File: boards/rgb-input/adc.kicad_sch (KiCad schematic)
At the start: 1 part, among them U2 MCP3208

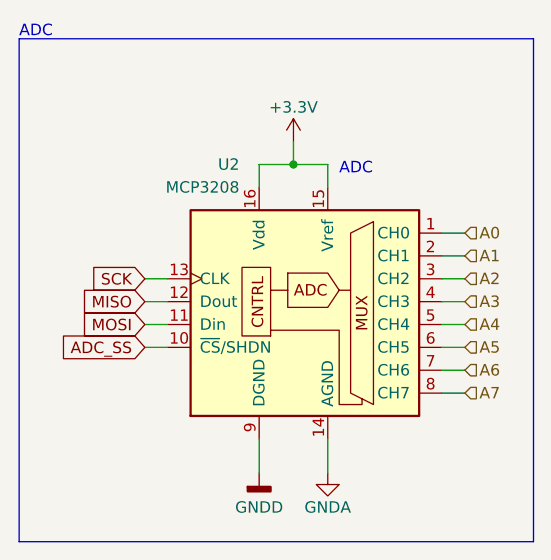
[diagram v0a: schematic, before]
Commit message: new rgb input board is starting to look very nice.
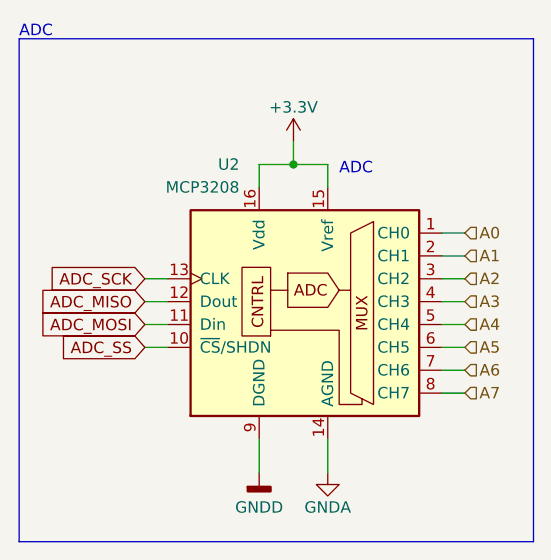
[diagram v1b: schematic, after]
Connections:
- net MISO renamed ADC_MISO
- net MOSI renamed ADC_MOSI
- net SCK renamed ADC_SCK
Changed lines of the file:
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@@
     (effects (font (size 1.27 1.27)) (justify left bottom))
   )
-  (global_label "SCK" (shape input) (at 118.11 85.09 180) (fields_autoplaced)
+  (global_label "ADC_SCK" (shape input) (at 118.11 85.09 180) (fields_autoplaced)
     (effects (font (size 1.27 1.27)) (justify right))
-    (property "Intersheetrefs" "${INTERSHEET_REFS}" (at 111.3753 85.09 0)
+    (property "Intersheetrefs" "${INTERSHEET_REFS}" (at 106.7791 85.09 0)
       (effects (font (size 1.27 1.27)) (justify right) hide)
     )
   )
-  (global_label "MISO" (shape input) (at 118.11 87.63 180) (fields_autoplaced)
+  (global_label "ADC_MISO" (shape input) (at 118.11 87.63 180) (fields_autoplaced)
     (effects (font (size 1.27 1.27)) (justify right))
-    (property "Intersheetrefs" "${INTERSHEET_REFS}" (at 110.5286 87.63 0)
+    (property "Intersheetrefs" "${INTERSHEET_REFS}" (at 105.9324 87.63 0)
       (effects (font (size 1.27 1.27)) (justify right) hide)
     )
   )
-  (global_label "MOSI" (shape input) (at 118.11 90.17 180) (fields_autoplaced)
+  (global_label "ADC_MOSI" (shape input) (at 118.11 90.17 180) (fields_autoplaced)
     (effects (font (size 1.27 1.27)) (justify right))
-    (property "Intersheetrefs" "${INTERSHEET_REFS}" (at 110.5286 90.17 0)
+    (property "Intersheetrefs" "${INTERSHEET_REFS}" (at 105.9324 90.17 0)
       (effects (font (size 1.27 1.27)) (justify right) hide)
     )

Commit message: reannotated and did some more cleanup.  almost ready
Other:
- company: (none) -> github.com/hoeken/yarrboard
- title: (none) -> RGB Input Board
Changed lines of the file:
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@@
 (kicad_sch (version 20230121) (generator eeschema)
   (paper "A4")
+  (title_block
+    (title "RGB Input Board")
+    (rev "B")
+    (company "github.com/hoeken/yarrboard")
+    (comment 1 "Open Source Hardware")
+  )
   (junction (at 134.62 72.39) (diameter 0) (color 0 0 0 0)
   )
@@
         )
         (path "/c83c6236-96e9-46ad-9d7a-9e2efa4a7966/b87f80e1-ecbd-4ee0-be26-4b252158928b"
-          (reference "#PWR07") (unit 1)
+          (reference "#PWR030") (unit 1)
         )
       )
@@
         )
         (path "/c83c6236-96e9-46ad-9d7a-9e2efa4a7966/b87f80e1-ecbd-4ee0-be26-4b252158928b"
-          (reference "#PWR057") (unit 1)
+          (reference "#PWR028") (unit 1)
         )
       )
@@
         )
         (path "/c83c6236-96e9-46ad-9d7a-9e2efa4a7966/b87f80e1-ecbd-4ee0-be26-4b252158928b"
-          (reference "#PWR06") (unit 1)
-        )
-      )
+          (reference "#PWR029") (unit 1)
+        )
+      )
